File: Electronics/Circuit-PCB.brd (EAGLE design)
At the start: 71.1 x 54.3 mm, 16 parts

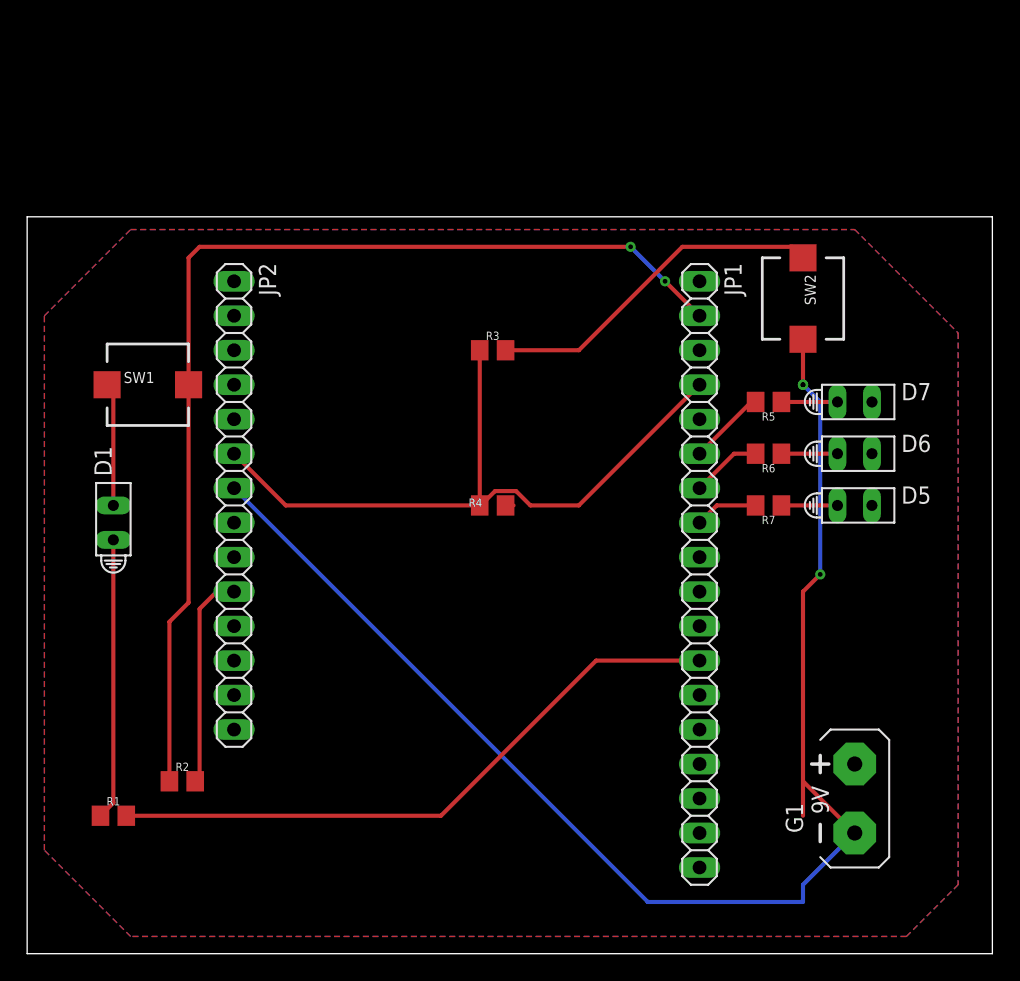
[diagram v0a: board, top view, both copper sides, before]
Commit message: Updated all electronics files
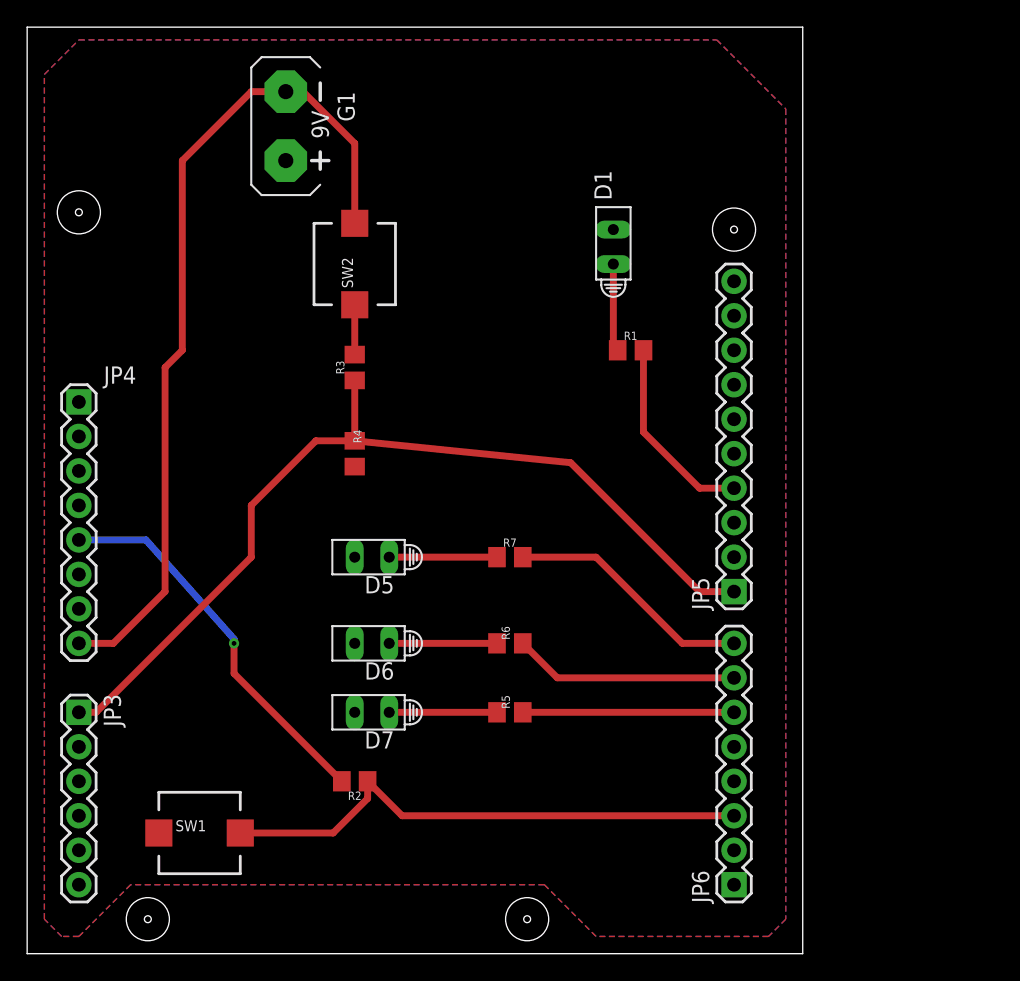
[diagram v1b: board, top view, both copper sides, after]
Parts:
- removed JP1: (no value), adafruit:1X18
- removed JP2: (no value), adafruit:1X14
- added JP3: (no value), arduino_jw:CONN-1X06
- added JP4, JP6: (no value), arduino_jw:CONN-1X08
- added JP5: ARDUINO_CONN-IO_HSIP, arduino_jw:CONN-1X10
- moved G1 64.9 mm to (19.1, 61.0), turned to 180 degrees
- moved R1 51.3 mm to (44.5, 44.5)
- moved D7 42.3 mm to (25.4, 17.8), turned to 180 degrees
- moved D1 42.1 mm to (43.2, 52.1)
- moved D6 38.2 mm to (25.4, 22.9), turned to 180 degrees
- moved D5 35.8 mm to (25.4, 29.2), turned to 180 degrees
- moved SW1 33.2 mm to (12.7, 8.89)
- moved SW2 33.1 mm to (24.1, 50.8), turned to 90 degrees
- moved R5 29.8 mm to (35.6, 17.8), turned to 0 degrees
- moved R6 23.6 mm to (35.6, 22.9), turned to 0 degrees
- moved R7 19.4 mm to (35.6, 29.2), turned to 0 degrees
- moved R2 12.7 mm to (24.1, 12.7), turned to 180 degrees
- moved R4 10.9 mm to (24.1, 36.8), turned to 90 degrees
- moved R3 10.2 mm to (24.1, 43.2), turned to 90 degrees
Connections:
- net GND: now also JP5.7; no longer JP1.15
- net N$1: now also JP4.8; no longer JP2.7
- net N$10: now also JP6.7; no longer JP1.7
- net N$11: now also JP6.8; no longer JP1.8
- net N$13: now also JP3.1, JP5.1; no longer JP1.4, JP2.6
- net N$14: now also JP4.5; no longer JP2.10
- net N$2: now also JP5.4; no longer JP1.12
- net N$5: now also JP6.3; no longer JP1.2
- net N$8: now also JP6.6; no longer JP1.6
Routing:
- net N$1: track 102.7 -> 62.5 mm, vias 3 -> 0
- net N$5: track 79.5 -> 39.7 mm, vias 2 -> 0
- net N$2: track 47.0 -> 14.4 mm
- net N$6: track 25.4 -> 3.67 mm
- net N$13: track 51.9 -> 67.2 mm
- net N$3: track 20.7 -> 6.48 mm
- net N$11: track 4.66 -> 18.2 mm
- net N$14: track 15.9 -> 28.5 mm, vias 0 -> 1
- net N$10: track 5.18 -> 16.6 mm
- net N$8: track 5.71 -> 15.6 mm
- net GND: track 9.67 -> 0.00 mm
- net N$9: track 4.13 -> 7.94 mm
- net N$7: track 4.13 -> 7.94 mm
- net N$4: track 4.13 -> 7.94 mm
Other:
- board size 71.1 x 54.3 mm -> 57.1 x 68.2 mm
